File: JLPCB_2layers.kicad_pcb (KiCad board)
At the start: 2 copper layers, 64 parts, among them J1 NS Connector, J2 EW Connector, J3 Control Logic Connector, J4 +5V, SW1 RST, SW2 OVR, SW3 EN, U1 SM420561N, U2 SM420561N, U3 LM1117DT-3.3

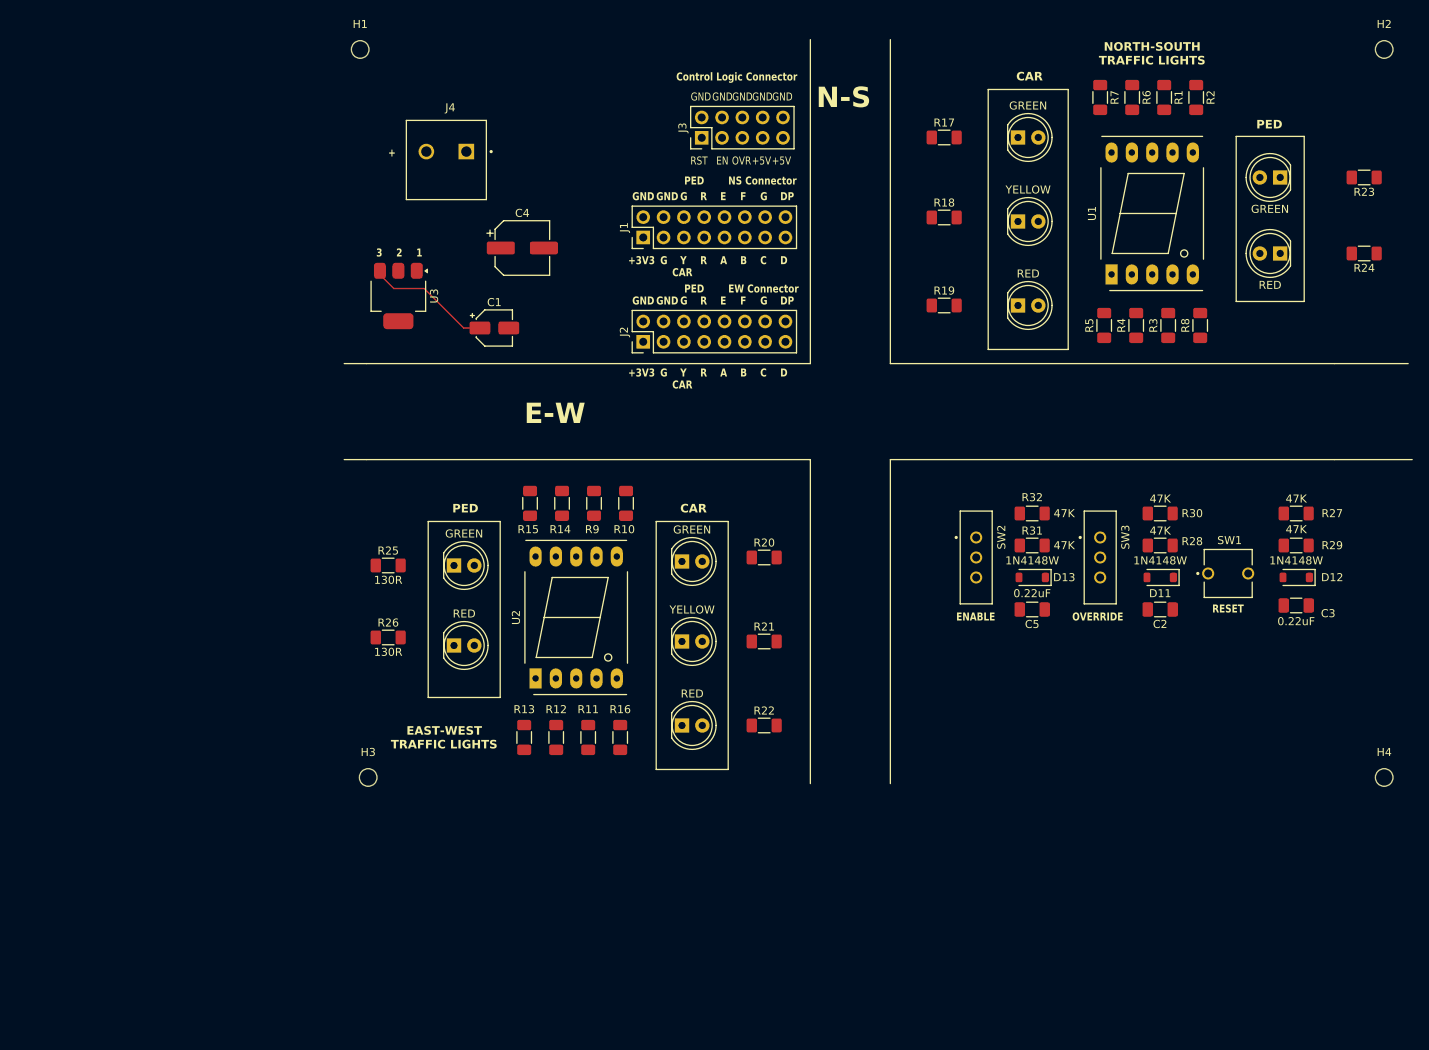
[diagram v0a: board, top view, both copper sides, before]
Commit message: Finalized and finished PCB
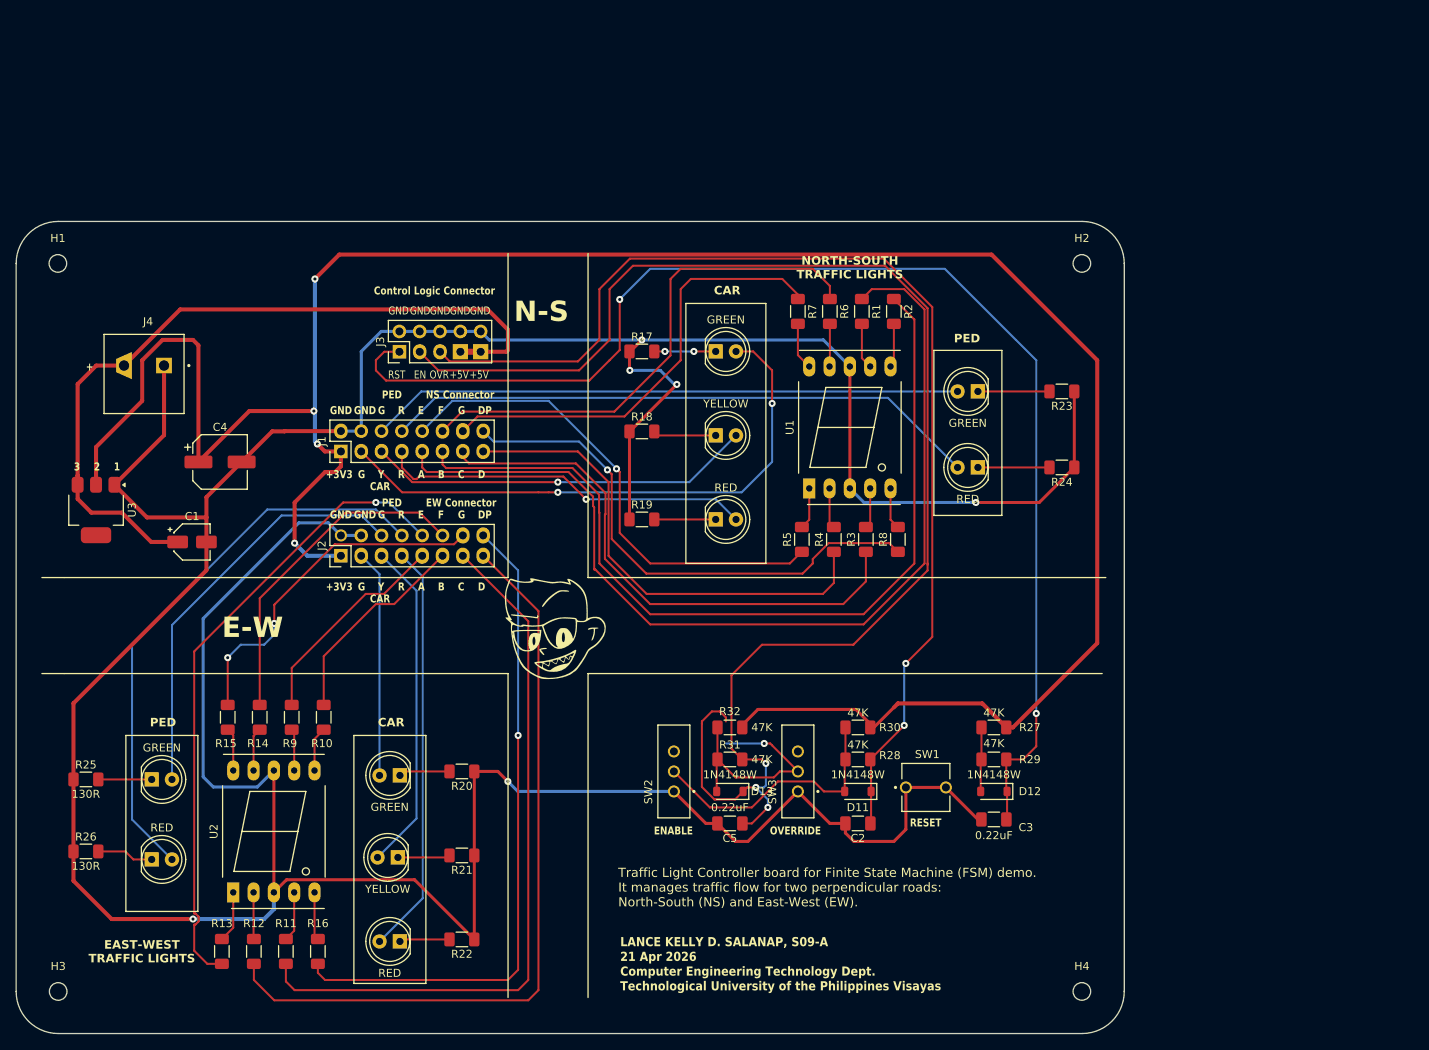
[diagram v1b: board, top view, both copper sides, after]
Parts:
- added G***: LOGO, my_footprints:Lance_logo_15x15mm, F.Cu at (142.7, 98.2)
- moved H3 47.1 mm to (81.2, 143.8)
- moved C1 46.3 mm to (98.0, 87.6)
- moved C4 46.3 mm to (101.5, 77.6)
- moved H1 46.3 mm to (81.2, 52.7)
- moved J4 46.3 mm to (92.0, 65.5)
- moved R11 46.3 mm to (109.7, 138.7)
- moved R12 46.3 mm to (105.7, 138.7)
- moved R13 46.3 mm to (101.7, 138.7)
- moved R16 46.3 mm to (113.7, 138.7)
- moved R25 46.3 mm to (84.7, 117.2)
- moved R26 46.3 mm to (84.7, 126.2)
- moved C2 46.3 mm to (181.2, 122.7)
- moved C3 46.3 mm to (198.2, 122.2)
- moved C5 46.3 mm to (165.2, 122.7)
- moved D11 46.3 mm to (181.2, 118.7)
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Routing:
- net GND: track 0.00 -> 498.6 mm, vias 0 -> 6
- net /+3.3V: track 0.00 -> 296.6 mm, vias 0 -> 4
- net /EN: track 0.00 -> 184.9 mm, vias 0 -> 3
- net /RST: track 0.00 -> 162.3 mm, vias 0 -> 2
- net /OVR: track 0.00 -> 141.5 mm, vias 0 -> 2
- net /NS_HEX_A: track 0.00 -> 122.5 mm
- net /NS_HEX_B: track 0.00 -> 110.1 mm
- net /EW_HEX_D: track 0.00 -> 96.3 mm
- net /EW_HEX_C: track 0.00 -> 89.9 mm
- net /+5V: track 15.8 -> 100.1 mm
- net /EW_HEX_DP: track 0.00 -> 83.2 mm, vias 0 -> 1
- net /EW_HEX_E: track 0.00 -> 80.1 mm, vias 0 -> 1
- net /NSP_RED: track 0.00 -> 74.8 mm
- net /NSP_GRN: track 0.00 -> 74.1 mm
- net /NSC_GRN: track 0.00 -> 72.1 mm, vias 0 -> 2
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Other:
- board outline added: 138.5 x 101.5 mm
- board text added: "LANCE KELLY D. SALANAP, S09-A 21 Apr 2026 Computer Engineering Technology Dept. Technological University of the Philippines Visayas"
- board text added: "Traffic Light Controller board for Finite State Machine (FSM) demo. It manages traffic flow for two perpendicular roads: North-South (NS) and East-West (EW)."

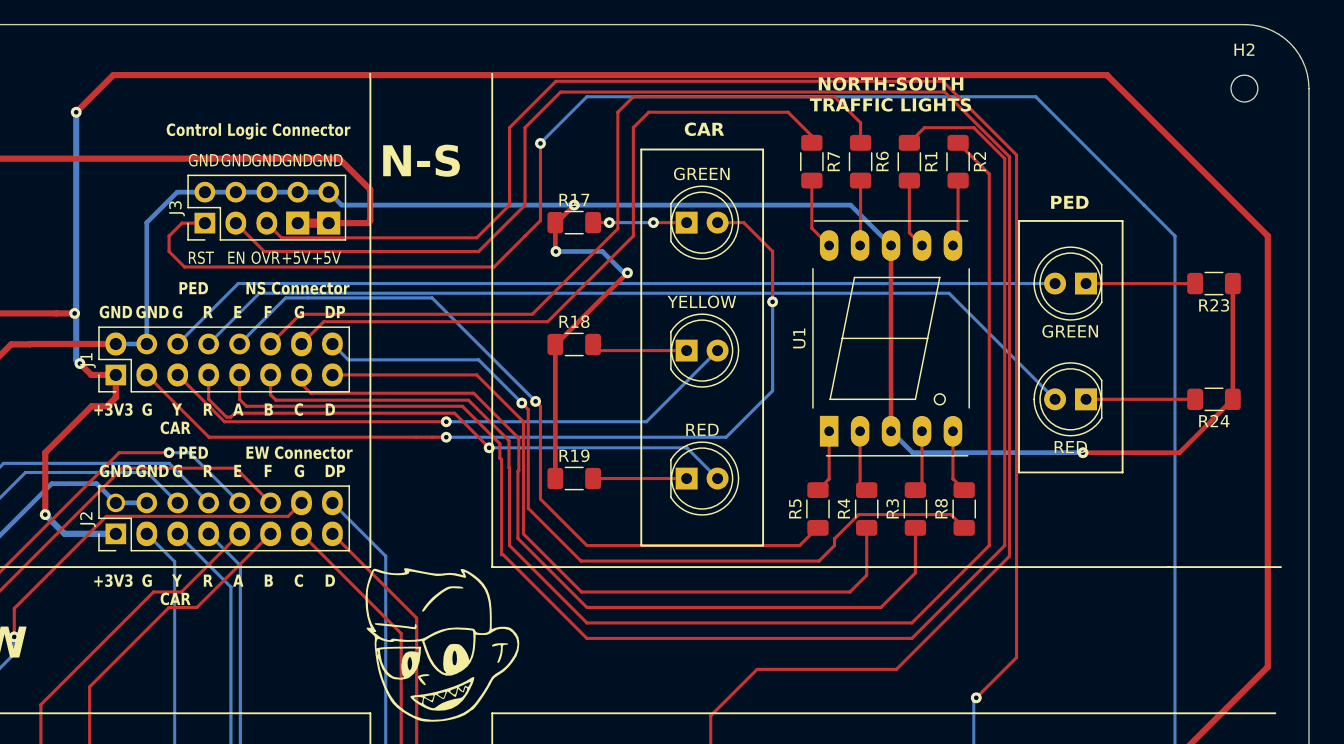
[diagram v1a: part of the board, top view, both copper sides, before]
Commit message: Finishing up and finalize PCB
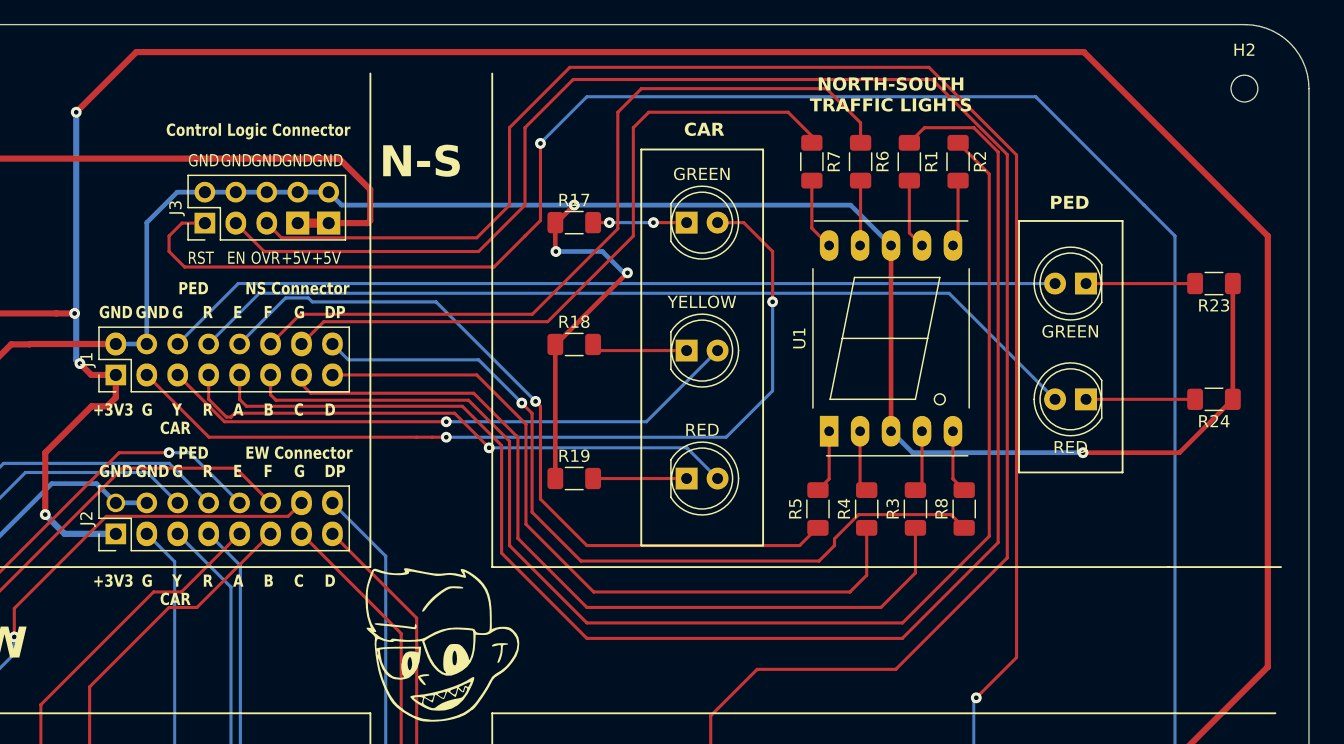
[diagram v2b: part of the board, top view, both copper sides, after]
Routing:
- net /+3.3V: track 296.6 -> 298.2 mm
- net /NS_HEX_A: track 122.5 -> 121.5 mm
- net /OVR: track 141.5 -> 142.4 mm
- net /EN: track 184.9 -> 185.6 mm
- net /NS_HEX_D: track 61.1 -> 60.5 mm
- net /NS_HEX_F: track 65.0 -> 65.5 mm
